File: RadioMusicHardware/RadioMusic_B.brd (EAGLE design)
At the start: 107 x 19.5 mm, 47 parts, among them IC1 REG1117, IC4 TL074, SW1 KMR2, X2 32.768, X3 microUSB

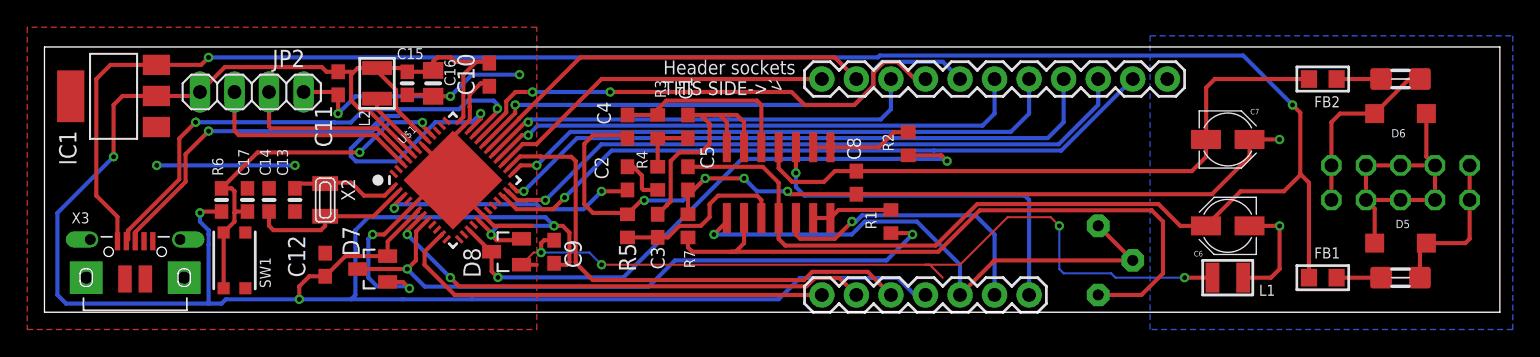
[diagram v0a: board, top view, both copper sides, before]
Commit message: Rev A of MTM Brain board.
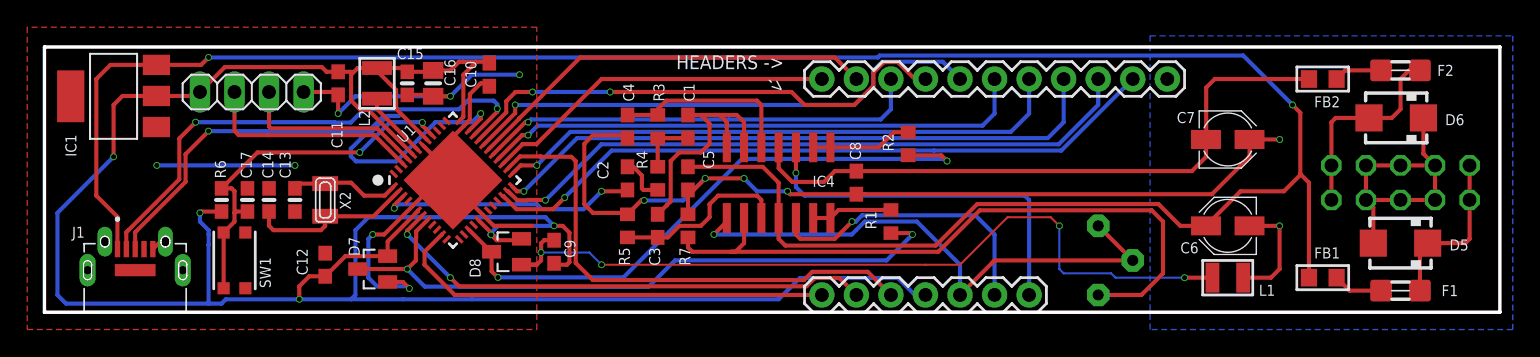
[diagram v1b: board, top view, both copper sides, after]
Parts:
- removed U$1: ATSAMD51G19A, SparkFun-IC-Microcontroller:QFN-48
- removed X3: microUSB, microbuilder:4UCONN_20329_V2
- added J1: UJ2-MIBH2-4-SMT-TR, UJ2-MIBH2-4-SMT-TR:CUI_UJ2-MIBH2-4-SMT-TR
- added U1: ATSAMD51G19A, SparkFun-IC-Microcontroller:QFN-48
- C10, C11, C12, C9: device adafruit:C0603 -> rcl:C0603
- C16: value 10uF -> 10u
- C17: value 1uF -> 1u
- D5, D6: value 1N4001 -> S1M; device diode:SOD123 -> diode:SMA
- moved F1 0.95 mm to (99.7, 1.59)
- moved F2 0.64 mm to (99.7, 17.8)
- moved D6 0.45 mm to (99.4, 14.3)
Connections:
- net !RESET: now also U1.40; no longer U$1.40
- net +12V: now also J1.1; no longer X3.VBUS
- net 3V3: now also U1.17, U1.36, U1.41, U1.44, U1.6; no longer U$1.17, U$1.36, U$1.41, U$1.44, U$1.6
- net CHANNEL_POT: now also U1.11; no longer U$1.11
- net D+: now also J1.3, U1.34; no longer U$1.34, X3.D+
- net D-: now also J1.2, U1.33; no longer U$1.33, X3.D-
- net DAC: now also U1.3; no longer U$1.3
- net DGND: now also J1.5, J1.SH1, J1.SH2, J1.SH3, J1.SH4, J1.SH5, U1.18, U1.35, U1.42, U1.5, U1.EP; no longer U$1.18, U$1.35, U$1.42, U$1.5, U$1.EP, X3.BASE@1, X3.BASE@2, X3.GND, X3.SPRT@1, X3.SPRT@2, X3.SPRT@3, X3.SPRT@4
- net LED1: now also U1.22; no longer U$1.22
- net LED2: now also U1.23; no longer U$1.23
- net LED3: now also U1.24; no longer U$1.24
- net LED4: now also U1.25; no longer U$1.25
- net LED_RESET: now also U1.30; no longer U$1.30
- net MISO: now also U1.27; no longer U$1.27
- net MOSI: now also U1.28; no longer U$1.28
- net N$11: now also U1.43; no longer U$1.43
- net N$13: now also U1.39; no longer U$1.39
- net N$8: now also U1.1; no longer U$1.1
- net N$9: now also U1.2; no longer U$1.2
- net PIN20/A6: now also U1.15; no longer U$1.15
- net PIN22/A8: now also U1.8; no longer U$1.8
- net RESET_CV: now also U1.32; no longer U$1.32
- net RESET_SW: now also U1.31; no longer U$1.31
- net SCLK: now also U1.26; no longer U$1.26
- net SS: now also U1.29; no longer U$1.29
- net SWCLK: now also U1.45; no longer U$1.45
- net SWDIO: now also U1.46; no longer U$1.46
- net TIME_POT: now also U1.7; no longer U$1.7
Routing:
- net DGND: track 119.3 -> 128.4 mm
- net -12V_INLET: track 13.5 -> 15.1 mm
- net +12V_INLET: track 11.4 -> 12.3 mm
- net 3V3: track 187.4 -> 186.8 mm
- net D-: track 36.8 -> 37.4 mm
- net D+: track 42.6 -> 43.2 mm
- net +12V: track 169.3 -> 169.9 mm
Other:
- board text added: "3V3"
- board text added: "CLK"
- board text added: "Dec 2014 / Summer 2019 musicthing.co.uk CC-BY-SA"
- board text added: "GND"
- board text added: "HEADERS ->"
- board text added: "IO"
- board text added: "Inspired by: John Cage Don Buchla Akin Fernandez Stockhausen Nicholas Collins Max Neuhaus UbuWeb Resonance FM John Peel archive.org"
- board text added: "MTM Brain PCB Rev A Designed in London Tom Whitwell, Tom Armitage"
- board text added: "Thanks to: Paul Stoffregen, Steven Thonk, The Muff Wigglers Limor Fried, Albert van Dalen"
- board text removed: "<-AUDIO OUT"
- board text removed: "December 2014 musicthing.co.uk CC-BY-SA"
- board text removed: "Header sockets THIS SIDE->"
- board text removed: "Inspired by: John Cage Don Buchla Akin Fernandez Stockhausen Nicholas Collins Max Neuhaus UbuWeb Resonance FM John Peel archive.org Thanks to: Paul Stoffregen, Steven Thonk, The Muff Wigglers"
- board text removed: "Radio Music Back PCB Rev2 Designed in Herne Hill, London by Tom Whitwell"
- board text removed: "TEENSY 3.1"
- board text removed: "USB this end"
